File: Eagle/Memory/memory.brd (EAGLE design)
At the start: 100 x 100 mm, 61 parts

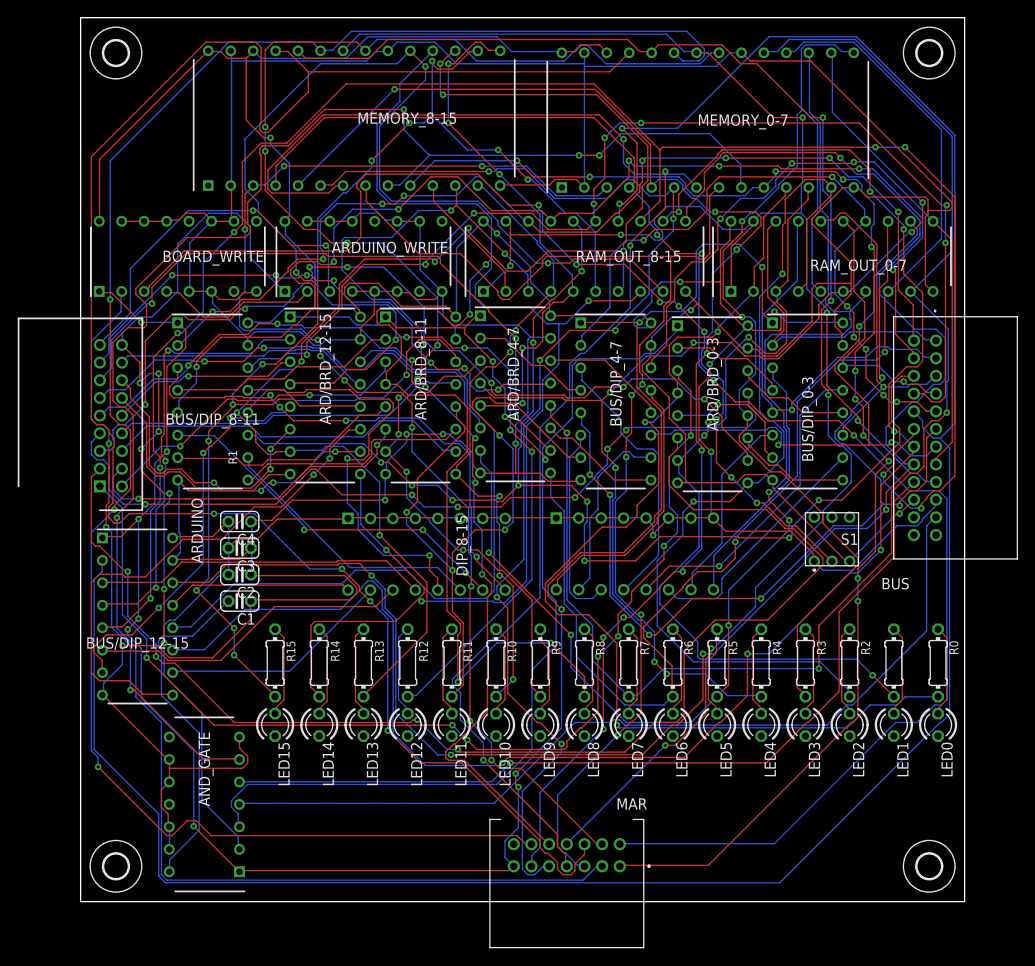
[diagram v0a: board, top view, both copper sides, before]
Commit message: added gerber files for ordering boards
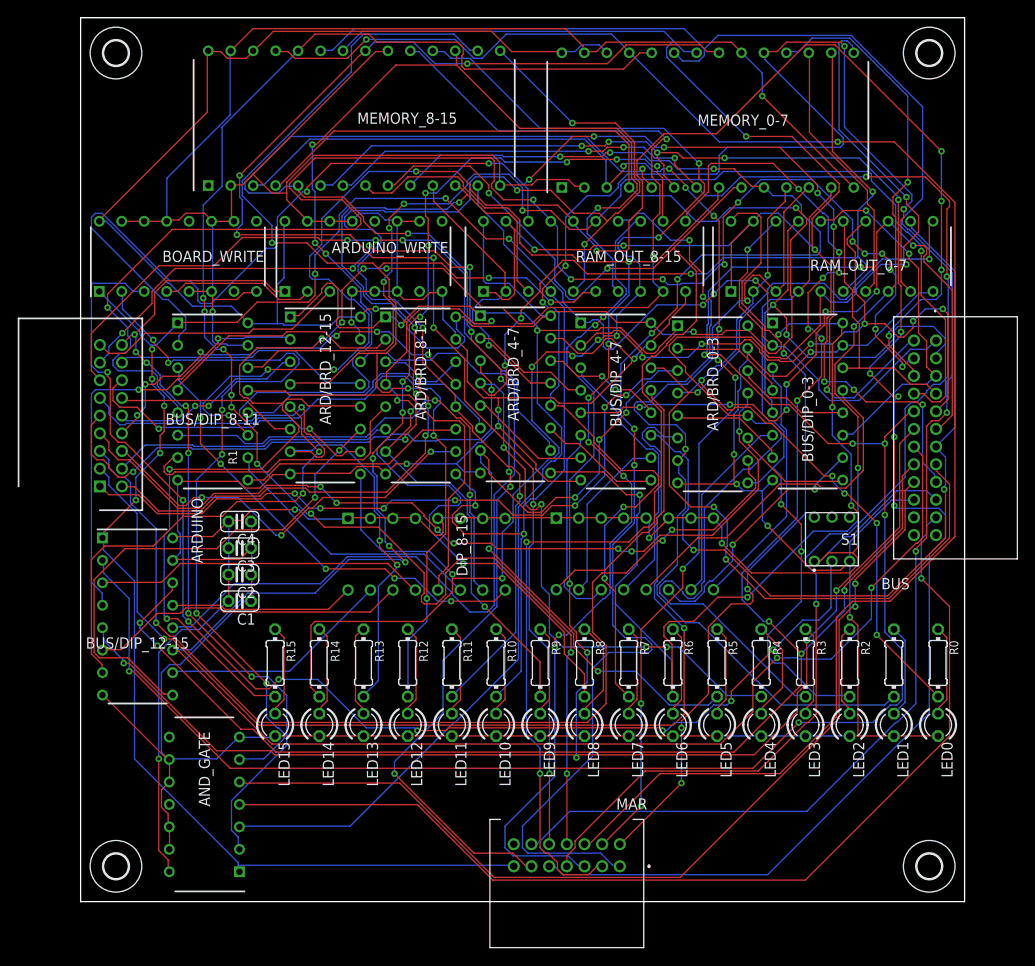
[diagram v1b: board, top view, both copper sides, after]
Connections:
- net GND: now also LED0.K, LED1.K, LED10.K, LED11.K, LED12.K, LED13.K, LED14.K, LED15.K, LED2.K, LED3.K, LED4.K, LED5.K, LED6.K, LED7.K, LED8.K, LED9.K
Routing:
- net B12: track 267.1 -> 192.4 mm, vias 2 -> 8
- net A1: track 221.1 -> 150.9 mm
- net GND: track 568.4 -> 637.2 mm, vias 7 -> 12
- net A4: track 141.4 -> 193.5 mm, vias 6 -> 10
- net B8: track 118.4 -> 162.8 mm
- net RAM0: track 122.2 -> 79.3 mm, vias 3 -> 6
- net ARD0: track 123.5 -> 80.7 mm
- net B10: track 134.9 -> 174.5 mm, vias 10 -> 9
- net B9: track 134.1 -> 173.2 mm, vias 7 -> 12
- net B14: track 193.4 -> 225.6 mm, vias 7 -> 13
- net B7: track 80.1 -> 110.5 mm, vias 3 -> 4
- net B5: track 111.0 -> 81.6 mm, vias 6 -> 7
- net RAM2: track 105.1 -> 77.0 mm
- net N$2: track 116.4 -> 140.8 mm
- net A6: track 176.6 -> 154.3 mm, vias 4 -> 5
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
